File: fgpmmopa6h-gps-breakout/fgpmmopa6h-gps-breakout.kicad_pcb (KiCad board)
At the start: 2 copper layers, 15 parts, among them J1 BREAKOUT, U1 MIC5365, U2 FGPMMOPA6H-GPS

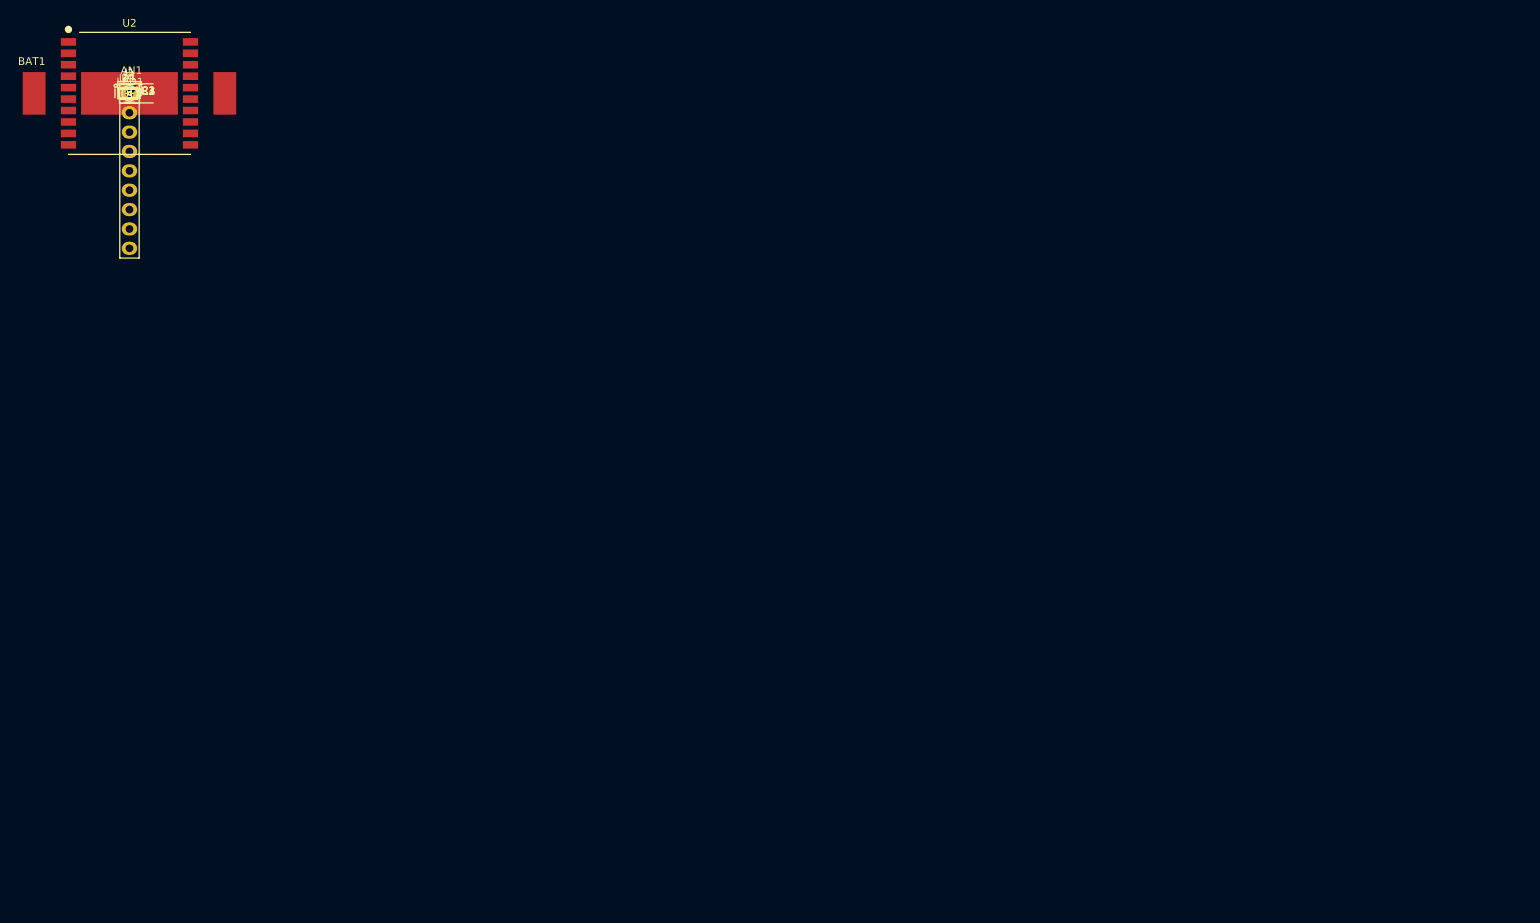
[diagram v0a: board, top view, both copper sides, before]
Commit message: Release FGPMMOPA6H GPS breakout v1.0
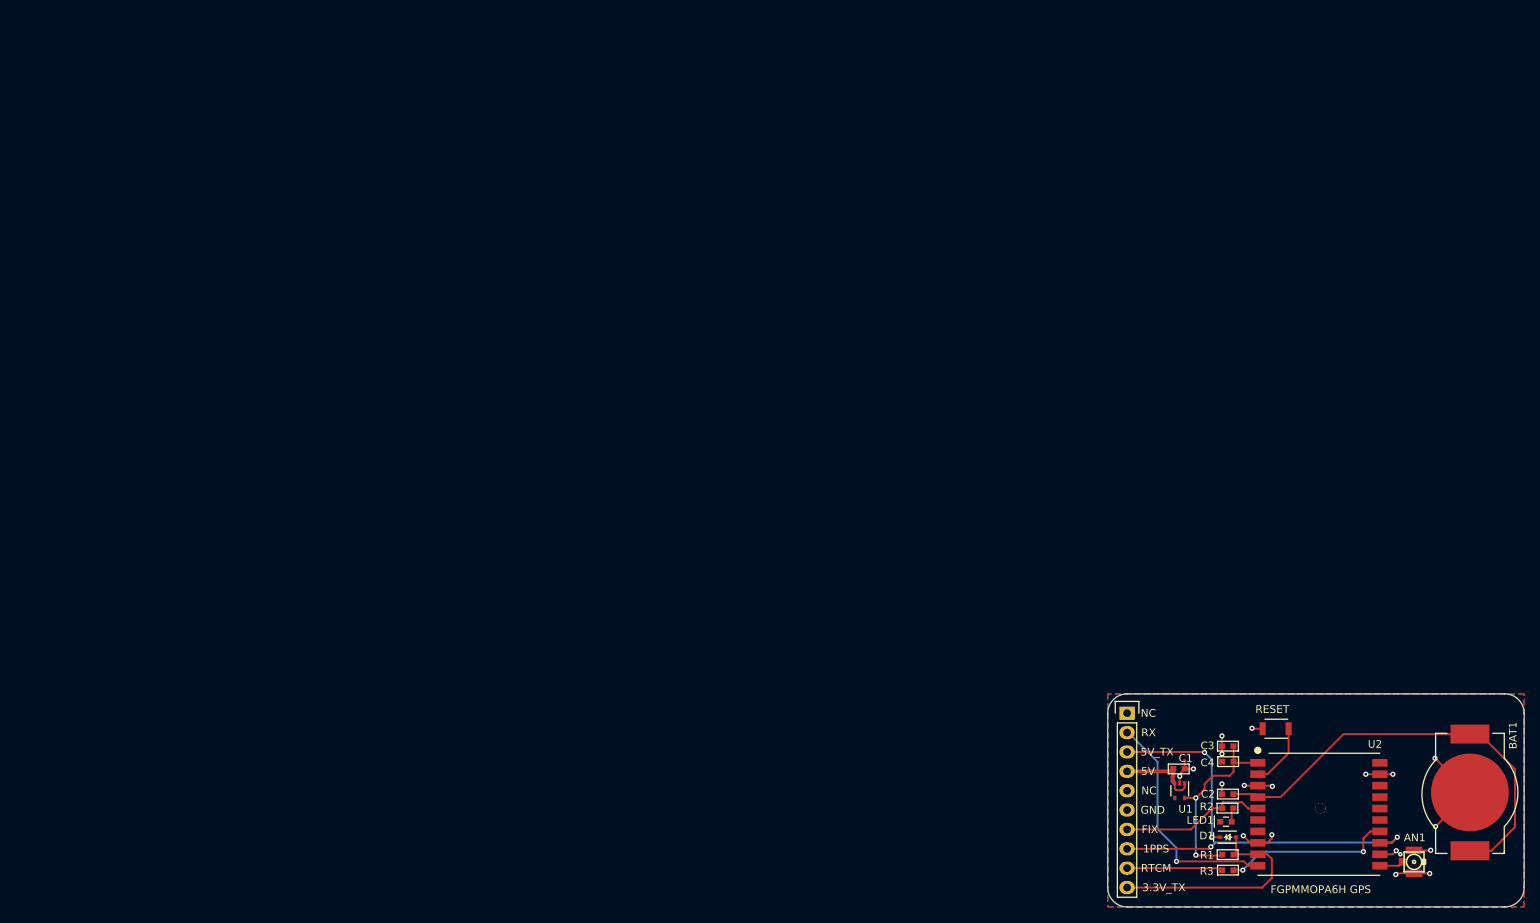
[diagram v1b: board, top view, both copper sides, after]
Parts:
- BAT1: footprint Wickerlib:BATT-HOLDER-STRAP-CR2032-BC-2003 -> Wickerlib:BATT-HOLDER-CR1220-BK-916
- J1: footprint Wickerlib:CONN-HEADER-STRAIGHT-P2.54MM-1x09 -> Wickerlib:CONN-HEADER-STRAIGHT-P2.54MM-1x10
- moved BAT1 198.2 mm to (175.8, 91.7), turned to 270 degrees
- moved AN1 196.3 mm to (168.4, 100.8)
- moved U2 182.4 mm to (156.0, 94.5)
- moved R3 176.4 mm to (144.0, 101.9), turned to 180 degrees
- moved R1 175.2 mm to (144.0, 99.8)
- moved D1 174.0 mm to (144.1, 97.5)
- moved S1 173.3 mm to (152.0, 83.3), turned to 180 degrees
- moved LED1 172.6 mm to (143.8, 95.5)
- moved R2 171.8 mm to (144.0, 93.7)
- moved C2 170.8 mm to (144.0, 91.9), turned to 180 degrees
- moved C4 168.6 mm to (144.0, 87.6), turned to 180 degrees
- moved C3 167.5 mm to (144.0, 85.6), turned to 180 degrees
- moved U1 165.3 mm to (137.7, 91.4), turned to 270 degrees
- moved C1 163.7 mm to (137.6, 88.6)
- moved J1 154.0 mm to (130.8, 81.3)
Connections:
- net /FTDI_TX renamed /5V_TX
- D1 pad 2: /GPS_RX -> /3.3V_TX
- J1 pad 1: /~FTDI_RESET -> (no net)
- J1 pad 2: /FTDI_RX -> /GPS_RX
- R1 pad 2: /GPS_RX -> /3.3V_TX
- S1 pad 1: /~FTDI_RESET -> /~RESET
- U2 pad 2: /~FTDI_RESET -> /~RESET
- U2 pad 9: /FTDI_RX -> /3.3V_TX
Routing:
- net /VBACKUP: track 0.00 -> 58.5 mm
- net GND: track 0.00 -> 43.7 mm, vias 0 -> 18
- net /1PPS: track 0.00 -> 38.7 mm, vias 0 -> 2
- net /GPS_RX: track 0.00 -> 30.6 mm, vias 0 -> 1
- net /3.3V_TX: track 0.00 -> 29.7 mm
- net +3V3: track 0.00 -> 25.9 mm, vias 0 -> 2
- net /5V_TX: track 0.00 -> 22.8 mm, vias 0 -> 2
- net /GPS_RTCM: track 0.00 -> 22.3 mm, vias 0 -> 2
- net /3D-FIX: track 0.00 -> 19.3 mm
- net /RTCM: track 0.00 -> 12.6 mm
- net +5V: track 0.00 -> 10.9 mm
- net /~RESET: track 0.00 -> 8.37 mm
- net Net-(AN1-PadSIG): track 0.00 -> 3.19 mm
- net Net-(LED1-Pad2): track 0.00 -> 1.87 mm
- added copper zone on B.Cu, net GND
- added copper zone on F.Cu, net GND
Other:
- board outline added: 54.6 x 27.9 mm
- net class Default: clearance 0.254 -> 0.1524
- rule trace_clearance: 0.254 -> 0.1524
- board text added: "1/10/17"
- board text added: "1PPS"
- board text added: "3.3V_TX"
- board text added: "5V"
- board text added: "5V_TX"
- board text added: "FGPMMOPA6H GPS"
- board text added: "FGPMMOPA6H GPS Breakout Board v1.0"
- board text added: "FGPMMOPA6H GPS Breakout Board v1.0 Assembly Diagram"
- board text added: "FIX"
- board text added: "GND"
- board text added: "NC"
- board text added: "RESET"
- board text added: "RTCM"
- board text added: "RX"
- board text added: "wickerbox.net"
